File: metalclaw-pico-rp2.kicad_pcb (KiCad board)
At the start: 4 copper layers, 21 x 51 mm, 75 parts, among them J1 USB_C_Receptacle_USB2.0_14P, J2 Conn_01x05, J3 Conn_02x05_Odd_Even, J4 Conn_Coaxial, SW1 SW_Push, SW2 SW_Push, U1 ESP32-S2, U2 MX25L3236FM2I-08G-TR, U3 APS6404L-3SQRx-SN, U4 RP2350B, U5 XC6220B331MR, Y1 XRCGB40M000F1S2FR0

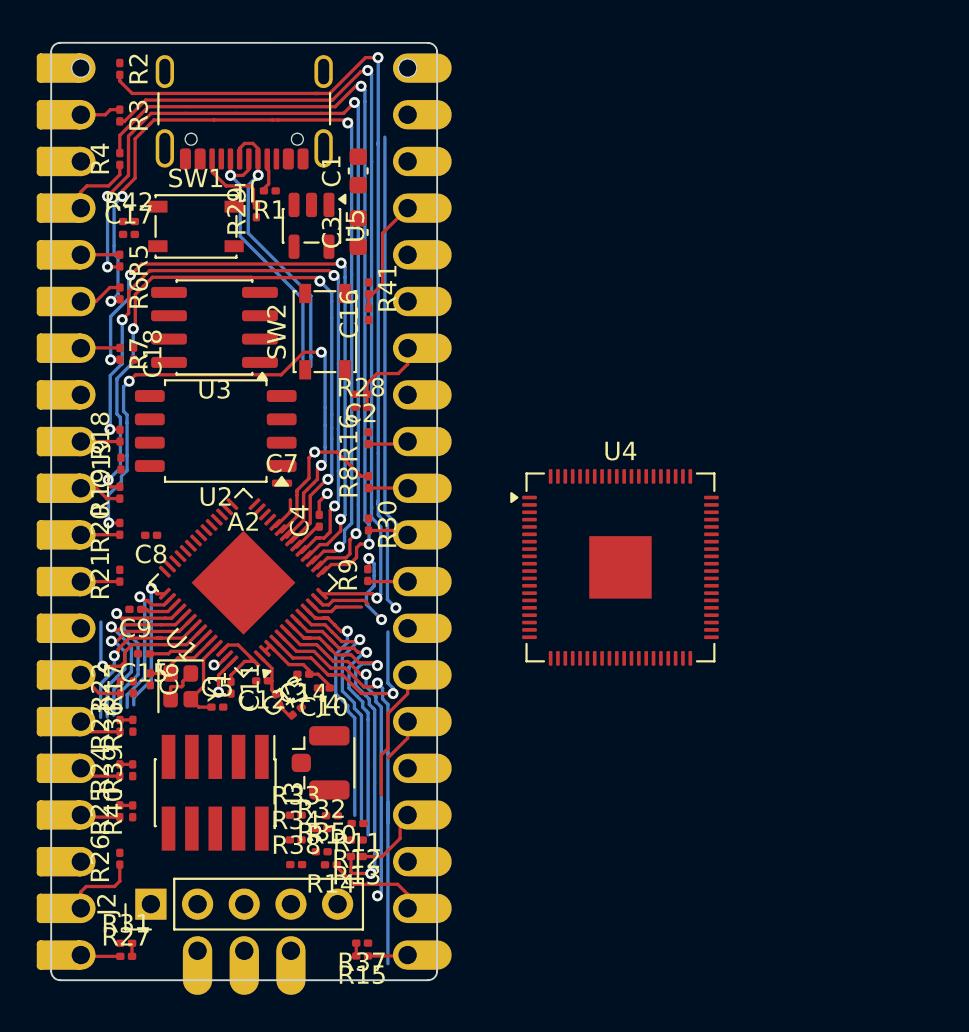
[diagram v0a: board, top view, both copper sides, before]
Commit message: Fill in BOM component details
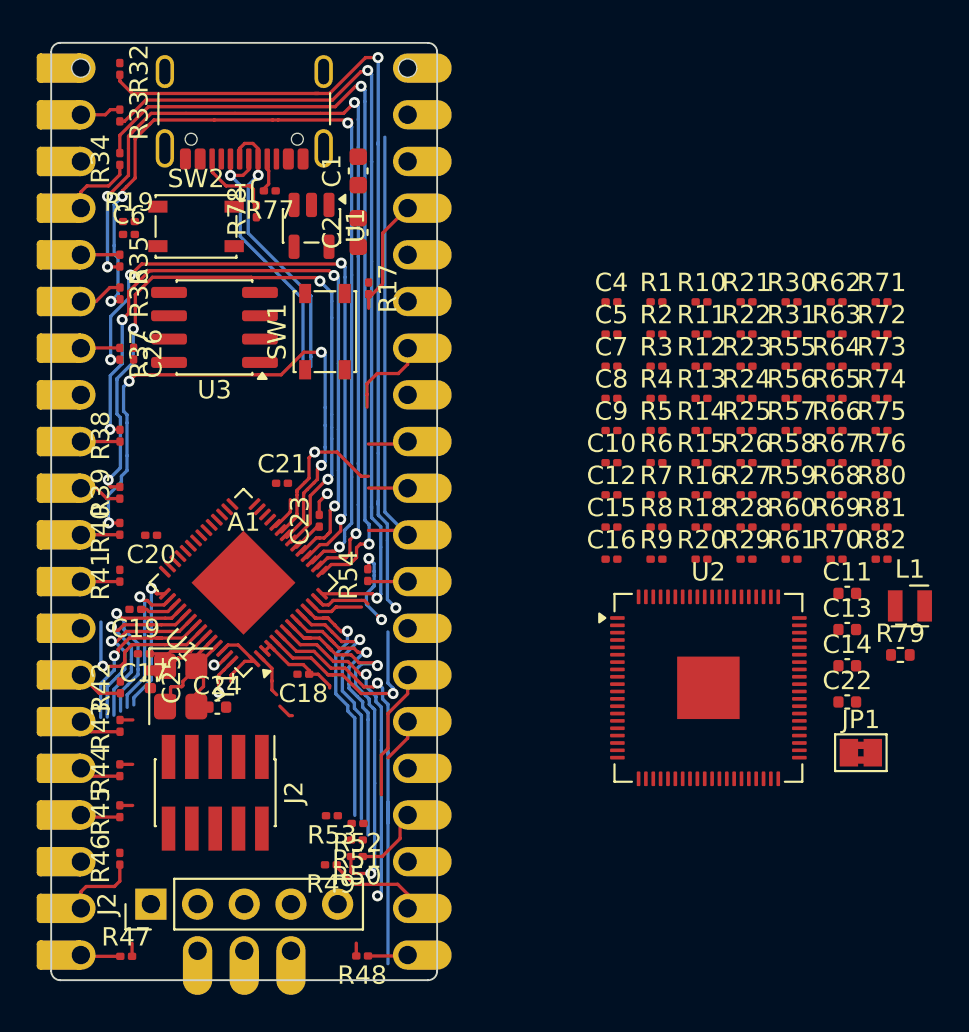
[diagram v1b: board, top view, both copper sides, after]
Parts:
- removed the C19 at (157.1, 96.3)
- removed the C2 at (170.2, 92.5)
- removed J4: Conn_Coaxial, Connector_Coaxial:U.FL_Hirose_U.FL-R-SMT-1_Vertical
- removed the R17 at (157.8, 108.4)
- removed the R32 at (168.0, 116.1)
- removed the R33 at (166.6, 115.4)
- removed the R34 at (166.6, 116.7)
- removed the R35 at (168.0, 117.4)
- removed the R36 at (157.8, 110.5)
- removed the R37 at (170.2, 122.3)
- removed the R38 at (166.6, 118.1)
- removed the R39 at (157.7, 112.9)
- removed the R40 at (157.7, 115.2)
- removed U4: RP2350B, Package_DFN_QFN:QFN-80-1EP_10x10mm_P0.4mm_EP3.4x3.4mm
- added C14: 4.7u, Capacitor_SMD:C_0402_1005Metric, F.Cu at (196.6, 107.3)
- added C15: 100n, Capacitor_SMD:C_0201_0603Metric, F.Cu at (183.8, 99.7)
- added C22: 4.7u, Capacitor_SMD:C_0402_1005Metric, F.Cu at (196.6, 109.2)
- added C4: 1u, Capacitor_SMD:C_0201_0603Metric, F.Cu at (183.8, 87.5)
- added C5: 1u, Capacitor_SMD:C_0201_0603Metric, F.Cu at (183.8, 89.2)
- added C7: 1u, Capacitor_SMD:C_0201_0603Metric, F.Cu at (183.8, 91.0)
- added C8: 1u, Capacitor_SMD:C_0201_0603Metric, F.Cu at (183.8, 92.7)
- added C9: 1u, Capacitor_SMD:C_0201_0603Metric, F.Cu at (183.8, 94.5)
- added JP1: Jumper_2_Bridged, Jumper:SolderJumper-2_P1.3mm_Bridged2Bar_Pad1.0x1.5mm, F.Cu at (197.4, 112.0)
- added R1: 5.1k, Resistor_SMD:R_0201_0603Metric, F.Cu at (186.2, 87.5)
- added R10: 5.1k, Resistor_SMD:R_0201_0603Metric, F.Cu at (188.7, 87.5)
- added R11: 5.1k, Resistor_SMD:R_0201_0603Metric, F.Cu at (188.7, 89.2)
- added R12: 5.1k, Resistor_SMD:R_0201_0603Metric, F.Cu at (188.7, 91.0)
- added R13: 5.1k, Resistor_SMD:R_0201_0603Metric, F.Cu at (188.7, 92.7)
- added R14: 5.1k, Resistor_SMD:R_0201_0603Metric, F.Cu at (188.7, 94.5)
- added R15: 5.1k, Resistor_SMD:R_0201_0603Metric, F.Cu at (188.7, 96.2)
- added R18: 5.1k, Resistor_SMD:R_0201_0603Metric, F.Cu at (188.7, 99.7)
- added R2: 5.1k, Resistor_SMD:R_0201_0603Metric, F.Cu at (186.2, 89.2)
- added R20: 5.1k, Resistor_SMD:R_0201_0603Metric, F.Cu at (188.7, 101.5)
- added R21: 5.1k, Resistor_SMD:R_0201_0603Metric, F.Cu at (191.1, 87.5)
- added R22: 5.1k, Resistor_SMD:R_0201_0603Metric, F.Cu at (191.1, 89.2)
- added R23: 5.1k, Resistor_SMD:R_0201_0603Metric, F.Cu at (191.1, 91.0)
- added R24: 5.1k, Resistor_SMD:R_0201_0603Metric, F.Cu at (191.1, 92.7)
- added R25: 5.1k, Resistor_SMD:R_0201_0603Metric, F.Cu at (191.1, 94.5)
- added R26: 5.1k, Resistor_SMD:R_0201_0603Metric, F.Cu at (191.1, 96.2)
- added R27: 5.1k, Resistor_SMD:R_0201_0603Metric, F.Cu at (191.1, 98.0)
- added R29: 5.1k, Resistor_SMD:R_0201_0603Metric, F.Cu at (191.1, 101.5)
- added R3: 5.1k, Resistor_SMD:R_0201_0603Metric, F.Cu at (186.2, 91.0)
- added R4: 5.1k, Resistor_SMD:R_0201_0603Metric, F.Cu at (186.2, 92.7)
- added R5: 5.1k, Resistor_SMD:R_0201_0603Metric, F.Cu at (186.2, 94.5)
- added R55: 220, Resistor_SMD:R_0201_0603Metric, F.Cu at (193.6, 91.0)
- added R56: 220, Resistor_SMD:R_0201_0603Metric, F.Cu at (193.6, 92.7)
- added R57: 220, Resistor_SMD:R_0201_0603Metric, F.Cu at (193.6, 94.5)
- added R58: 220, Resistor_SMD:R_0201_0603Metric, F.Cu at (193.6, 96.2)
- added R59: 220, Resistor_SMD:R_0201_0603Metric, F.Cu at (193.6, 98.0)
- added R6: 5.1k, Resistor_SMD:R_0201_0603Metric, F.Cu at (186.2, 96.2)
- added R60: 220, Resistor_SMD:R_0201_0603Metric, F.Cu at (193.6, 99.7)
- added R61: 220, Resistor_SMD:R_0201_0603Metric, F.Cu at (193.6, 101.5)
- added R62: 220, Resistor_SMD:R_0201_0603Metric, F.Cu at (196.0, 87.5)
- added R63: 220, Resistor_SMD:R_0201_0603Metric, F.Cu at (196.0, 89.2)
- added R64: 220, Resistor_SMD:R_0201_0603Metric, F.Cu at (196.0, 91.0)
- added R65: 220, Resistor_SMD:R_0201_0603Metric, F.Cu at (196.0, 92.7)
- added R66: 220, Resistor_SMD:R_0201_0603Metric, F.Cu at (196.0, 94.5)
- added R67: 220, Resistor_SMD:R_0201_0603Metric, F.Cu at (196.0, 96.2)
- added R68: 220, Resistor_SMD:R_0201_0603Metric, F.Cu at (196.0, 98.0)
- added R69: 220, Resistor_SMD:R_0201_0603Metric, F.Cu at (196.0, 99.7)
- added R7: 5.1k, Resistor_SMD:R_0201_0603Metric, F.Cu at (186.2, 98.0)
- added R70: 220, Resistor_SMD:R_0201_0603Metric, F.Cu at (196.0, 101.5)
- added R71: 220, Resistor_SMD:R_0201_0603Metric, F.Cu at (198.5, 87.5)
- added R72: 220, Resistor_SMD:R_0201_0603Metric, F.Cu at (198.5, 89.2)
- added R73: 220, Resistor_SMD:R_0201_0603Metric, F.Cu at (198.5, 91.0)
- added R74: 220, Resistor_SMD:R_0201_0603Metric, F.Cu at (198.5, 92.7)
- added R75: 220, Resistor_SMD:R_0201_0603Metric, F.Cu at (198.5, 94.5)
- added R76: 220, Resistor_SMD:R_0201_0603Metric, F.Cu at (198.5, 96.2)
- added R79: 33, Resistor_SMD:R_0402_1005Metric, F.Cu at (199.5, 106.7)
- added R80: 5.1k, Resistor_SMD:R_0201_0603Metric, F.Cu at (198.5, 98.0)
- added R81: 5.1k, Resistor_SMD:R_0201_0603Metric, F.Cu at (198.5, 99.7)
- added R82: 5.1k, Resistor_SMD:R_0201_0603Metric, F.Cu at (198.5, 101.5)
- added R9: 5.1k, Resistor_SMD:R_0201_0603Metric, F.Cu at (186.2, 101.5)
- C11: value 1u -> 100n; footprint Capacitor_SMD:C_0201_0603Metric -> Capacitor_SMD:C_0402_1005Metric
- C12: value C -> 1u
- C13: value C -> 4.7u; footprint Capacitor_SMD:C_0201_0603Metric -> Capacitor_SMD:C_0402_1005Metric
- C16: value 1u -> 100n
- C24: renamed from C5; value 6p -> 15p; footprint Capacitor_SMD:C_0201_0603Metric -> Capacitor_SMD:C_0402_1005Metric
- C25: renamed from C6; value 6p -> 15p; footprint Capacitor_SMD:C_0201_0603Metric -> Capacitor_SMD:C_0402_1005Metric
- L1: value L -> 3.3u; footprint Inductor_SMD:L_0201_0603Metric -> Inductor_SMD_Wurth:L_Wurth_WE-LQSH-2010
- R16, R28, R8: value 220 -> 5.1k
- U2: value MX25L3236FM2I-08G-TR -> RP2354B; footprint Package_SO:SOIC-8_5.3x5.3mm_P1.27mm -> Package_DFN_QFN:QFN-80-1EP_10x10mm_P0.4mm_EP3.4x3.4mm
- Y1: value XRCGB40M000F1S2FR0 -> ABM8-272-T3; footprint Crystal:Crystal_SMD_2016-4Pin_2.0x1.6mm -> Crystal:Crystal_SMD_3225-4Pin_3.2x2.5mm
- moved R31 49.1 mm to (193.6, 89.2)
- moved L1 34.8 mm to (200.0, 104.0), turned to 0 degrees
- moved C11 33.9 mm to (196.6, 103.3), turned to 0 degrees
- moved C13 30.3 mm to (196.6, 105.3), turned to 0 degrees
- moved U2 30.2 mm to (189.1, 108.5), turned to 0 degrees
- moved R30 26.0 mm to (193.6, 87.5), turned to 0 degrees
- moved R28 22.0 mm to (191.1, 99.7)
- moved C12 21.5 mm to (183.8, 98.0), turned to 0 degrees
- moved C10 19.9 mm to (183.8, 96.2), turned to 0 degrees
- moved C16 18.8 mm to (183.8, 101.5), turned to 0 degrees
- moved R16 18.4 mm to (188.7, 98.0), turned to 0 degrees
- moved R8 15.9 mm to (186.2, 99.7), turned to 0 degrees
- renumbered A2 to A1, C15 to C17, C14 to C18, C9 to C19, C3 to C2, C8 to C20, C7 to C21, C4 to C23, C18 to C26, C17 to C6, J3 to J2, R41 to R17, R42 to R19, R2 to R32, R3 to R33, R4 to R34, R5 to R35, R6 to R36, R7 to R37, R18 to R38, R19 to R39, R20 to R40, R21 to R41, R22 to R42, R23 to R43, R24 to R44, R25 to R45, R26 to R46, R27 to R47, R15 to R48, R14 to R49, R13 to R50, R12 to R51, R11 to R52, R10 to R53, R9 to R54, R1 to R77, R29 to R78, SW2 to SW1, SW1 to SW2, U5 to U1
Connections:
- A1 pad 1: Net-(A2-GPIO0) -> /GP0
- A1 pad 10: Net-(A2-GPIO7) -> /GP7
- A1 pad 11: Net-(A2-GPIO8) -> /GP8
- A1 pad 12: Net-(A2-GPIO9) -> /GP9
- A1 pad 14: Net-(A2-GPIO10) -> /GP10
- A1 pad 15: Net-(A2-GPIO11) -> /GP11
- A1 pad 16: Net-(A2-GPIO12) -> /GP12
- A1 pad 17: Net-(A2-GPIO13) -> /GP13
- A1 pad 19: Net-(A2-GPIO14) -> /GP14
- A1 pad 2: Net-(A2-GPIO1) -> /GP1
- A1 pad 20: Net-(A2-GPIO15) -> /GP15
- A1 pad 21: Net-(A2-GPIO16) -> /GP16
- A1 pad 22: Net-(A2-GPIO17) -> /GP17
- A1 pad 24: Net-(A2-GPIO18) -> /GP18
- A1 pad 25: Net-(A2-GPIO19) -> /GP19
- A1 pad 26: Net-(A2-GPIO20) -> /GP20
- A1 pad 27: Net-(A2-GPIO21) -> /GP21
- A1 pad 29: Net-(A2-GPIO22) -> /GP22
- A1 pad 31: Net-(A2-GPIO26_ADC0) -> Net-(A1-GPIO26_ADC0)
- A1 pad 32: Net-(A2-GPIO27_ADC1) -> Net-(A1-GPIO27_ADC1)
- A1 pad 33: GND -> Net-(A1-AGND)
- A1 pad 34: /GP28 -> Net-(A1-GPIO28_ADC2)
- A1 pad 35: +3V3 -> unconnected-(A1-ADC_VREF-Pad35)
- A1 pad 36: unconnected-(A2-3V3-Pad36) -> +3.3VP
- A1 pad 39: unconnected-(A2-VSYS-Pad39) -> VS
- A1 pad 4: Net-(A2-GPIO2) -> /GP2
- A1 pad 40: VBUS -> unconnected-(A1-VBUS-Pad40)
- A1 pad 5: Net-(A2-GPIO3) -> /GP3
- A1 pad 6: Net-(A2-GPIO4) -> /GP4
- A1 pad 7: Net-(A2-GPIO5) -> /GP5
- A1 pad 9: Net-(A2-GPIO6) -> /GP6
- C10 pad 1: +3V3 -> GND
- C10 pad 2: GND -> Net-(C10-Pad2)
- C11 pad 1: +3V3 -> GND
- C11 pad 2: GND -> Net-(U2-VREG_AVDD)
- C12 pad 1: Net-(U1-LNA_IN) -> GND
- C12 pad 2: GND -> +3V3
- C13 pad 1: Net-(J4-In) -> GND
- C13 pad 2: GND -> +3V3
- C16 pad 1: Net-(C16-Pad1) -> GND
- C16 pad 2: /3V3_EN -> +3V3
- C17 pad 1: +3V3 -> GND
- C17 pad 2: GND -> +3V3
- C18 pad 1: +3V3 -> GND
- C18 pad 2: GND -> +3V3
- C19 pad 1: +3V3 -> GND
- C19 pad 2: GND -> +3V3
- C20 pad 1: +3V3 -> GND
- C20 pad 2: GND -> +3V3
- C21 pad 1: +3V3 -> GND
- C21 pad 2: GND -> Net-(U2-VREG_FB)
- C23 pad 1: +3V3 -> GND
- C23 pad 2: GND -> +3V3
- C24 pad 1: Net-(U1-XTAL_P) -> Net-(U2-XIN)
- C25 pad 1: Net-(U1-XTAL_N) -> GND
- C25 pad 2: GND -> Net-(U2-XOUT)
- C26 pad 1: GND -> +3V3
- C26 pad 2: VDD -> GND
- C6 pad 1: Net-(C17-Pad1) -> GND
- J1 pad A6: /USB_D+ -> Net-(J1-D+-PadA6)
- J1 pad A7: /USB_D- -> Net-(J1-D--PadA7)
- J1 pad B6: /USB_D+ -> Net-(J1-D+-PadA6)
- J1 pad B7: /USB_D- -> Net-(J1-D--PadA7)
- J1 pad S1: unconnected-(J1-SHIELD-PadS1) -> GND
- J2 pad 10: unconnected-(J3-Pin_10-Pad10) -> /RESET
- J2 pad 2: /MTMS -> Net-(J2-Pin_2)
- J2 pad 4: /MTCK -> Net-(J2-Pin_4)
- J2 pad 6: /MTDO -> unconnected-(J2-Pin_6-Pad6)
- J2 pad 7: GND -> unconnected-(J2-Pin_7-Pad7)
- J2 pad 8: /MTDI -> unconnected-(J2-Pin_8-Pad8)
- L1 pad 1: Net-(U1-LNA_IN) -> Net-(U2-VREG_FB)
- L1 pad 2: Net-(J4-In) -> Net-(U2-VREG_LX)
- R16 pad 1: Net-(A2-GPIO27_ADC1) -> +3.3VP
- R16 pad 2: /GP27 -> /GP8
- R17 pad 2: /3V3_EN -> /BOOTSEL
- R28 pad 1: Net-(U1-GPIO21) -> /GP16
- R28 pad 2: /GP28 -> +3.3VP
- R30 pad 1: GND -> /GP27
- R30 pad 2: /RUN -> Net-(C9-Pad2)
- R31 pad 1: GND -> /GP28
- R31 pad 2: /GP15 -> Net-(C10-Pad2)
- R32 pad 1: Net-(A2-GPIO0) -> /GP3
- R32 pad 2: /GP0 -> Net-(U2-GPIO0)
- R33 pad 1: Net-(A2-GPIO1) -> /3V3_EN
- R33 pad 2: /GP1 -> Net-(U2-GPIO1)
- R34 pad 1: Net-(A2-GPIO2) -> /GP1
- R34 pad 2: /GP2 -> Net-(U2-GPIO2)
- R35 pad 1: Net-(A2-GPIO3) -> /GP0
- R35 pad 2: /GP3 -> Net-(U2-GPIO3)
- R36 pad 1: Net-(A2-GPIO4) -> /GP0
- R36 pad 2: /GP4 -> Net-(U2-GPIO4)
- R37 pad 1: Net-(A2-GPIO5) -> /GP1
- R37 pad 2: /GP5 -> Net-(U2-GPIO5)
- R38 pad 1: Net-(A2-GPIO6) -> /GP2
- R38 pad 2: /GP6 -> Net-(U2-GPIO6)
- R39 pad 1: Net-(A2-GPIO7) -> /GP3
- R39 pad 2: /GP7 -> Net-(U2-GPIO7)
- R40 pad 1: Net-(A2-GPIO8) -> /GP7
- R40 pad 2: /GP8 -> Net-(U2-GPIO8)
- R41 pad 1: Net-(A2-GPIO9) -> /RUN
- R41 pad 2: /GP9 -> Net-(U2-GPIO9)
- R42 pad 1: Net-(A2-GPIO10) -> /GP5
- R42 pad 2: /GP10 -> Net-(U2-GPIO10)
- R43 pad 1: Net-(A2-GPIO11) -> /GP4
- R43 pad 2: /GP11 -> Net-(U2-GPIO11)
- R44 pad 1: Net-(A2-GPIO12) -> /GP4
- R44 pad 2: /GP12 -> Net-(U2-GPIO12)
- R45 pad 1: Net-(A2-GPIO13) -> /GP5
- R45 pad 2: /GP13 -> Net-(U2-GPIO13)
- R46 pad 1: Net-(A2-GPIO14) -> /GP6
- R46 pad 2: /GP14 -> Net-(U2-GPIO14)
- R47 pad 1: Net-(A2-GPIO15) -> /GP7
- R47 pad 2: /GP15 -> Net-(U2-GPIO15)
- R48 pad 1: Net-(A2-GPIO16) -> /GP11
- R48 pad 2: /GP16 -> Net-(U2-GPIO16)
- R49 pad 1: Net-(A2-GPIO17) -> /SWCLK
- R49 pad 2: /GP17 -> Net-(U2-GPIO17)
- R50 pad 1: Net-(A2-GPIO18) -> /GP9
- R50 pad 2: /GP18 -> Net-(U2-GPIO18)
- R51 pad 1: Net-(A2-GPIO19) -> /GP8
- R51 pad 2: /GP19 -> Net-(U2-GPIO19)
- R52 pad 1: Net-(A2-GPIO20) -> /GP8
- R52 pad 2: /GP20 -> Net-(U2-GPIO20)
- R53 pad 1: Net-(A2-GPIO21) -> /GP9
- R53 pad 2: /GP21 -> Net-(U2-GPIO21)
- R54 pad 1: Net-(A2-GPIO22) -> /GP10
- R54 pad 2: /GP22 -> Net-(U2-GPIO22)
- R8 pad 1: Net-(A2-GPIO26_ADC0) -> +3.3VP
- R8 pad 2: /GP26 -> /GP12
- SW1 pad 2: Net-(C16-Pad1) -> Net-(R80-Pad2)
- SW2 pad 2: Net-(C17-Pad1) -> /RESET
- U2 pad 1: Net-(U1-SPICS0) -> Net-(U2-GPIO4)
- U2 pad 2: Net-(U1-SPIQ) -> Net-(U2-GPIO5)
- U2 pad 3: Net-(U1-SPIWP) -> Net-(U2-GPIO6)
- U2 pad 4: GND -> Net-(U2-GPIO7)
- U2 pad 5: Net-(U1-SPID) -> +3V3
- U2 pad 6: Net-(U1-SPICLK) -> Net-(U2-GPIO8)
- U2 pad 7: Net-(U1-SPIHD) -> Net-(U2-GPIO9)
- U2 pad 8: VDD -> Net-(U2-GPIO10)
- U3 pad 1: Net-(U1-SPICS1) -> Net-(U2-GPIO47/ADC7)
- U3 pad 2: Net-(U1-SPIQ) -> Net-(U2-QSPI_SD1)
- U3 pad 3: Net-(U1-SPIWP) -> Net-(U2-QSPI_SD2)
- U3 pad 5: Net-(U1-SPID) -> Net-(U2-QSPI_SD0)
- U3 pad 6: Net-(U1-SPICLK) -> Net-(U2-QSPI_SCLK)
- U3 pad 7: Net-(U1-SPIHD) -> Net-(U2-QSPI_SD3)
- U3 pad 8: VDD -> +3V3
- Y1 pad 1: Net-(U1-XTAL_N) -> Net-(U2-XIN)
- Y1 pad 3: Net-(U1-XTAL_P) -> Net-(U2-XOUT)
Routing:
- net (no net): track 0.00 -> 52.2 mm
- net Net-(U2-GPIO0): track 0.00 -> 46.5 mm, vias 0 -> 2
- net /GP0: track 49.6 -> 3.10 mm, vias 2 -> 0
- net Net-(J1-D--PadA7): track 0.00 -> 15.3 mm, vias 0 -> 1
- net /USB_D-: track 15.3 -> 0.00 mm, vias 1 -> 0
- net Net-(J1-D+-PadA6): track 0.00 -> 14.6 mm, vias 0 -> 1
- net /USB_D+: track 14.6 -> 0.00 mm, vias 1 -> 0
- net /GP21: track 13.8 -> 20.9 mm
- net Net-(A2-GPIO21): track 7.11 -> 0.00 mm
- net Net-(A2-GPIO17): track 5.36 -> 0.00 mm
- net Net-(U2-GPIO22): track 0.00 -> 4.87 mm, vias 0 -> 2
- net /GP22: track 7.84 -> 2.98 mm, vias 2 -> 0
- net Net-(A1-GPIO28_ADC2): track 0.00 -> 4.80 mm
- net /GP28: track 4.80 -> 0.00 mm
- net Net-(A2-GPIO14): track 4.16 -> 0.00 mm
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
